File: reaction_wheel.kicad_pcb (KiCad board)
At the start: 2 copper layers, 55.7 x 65.5 mm, 33 parts, among them J1 QTH-030-01-L-D-A, J2 FTSH-105-01-L-DV, U1 TPS61379QWRTERQ1, U2 TPS62902RPJR, U8 STM32G474RETx

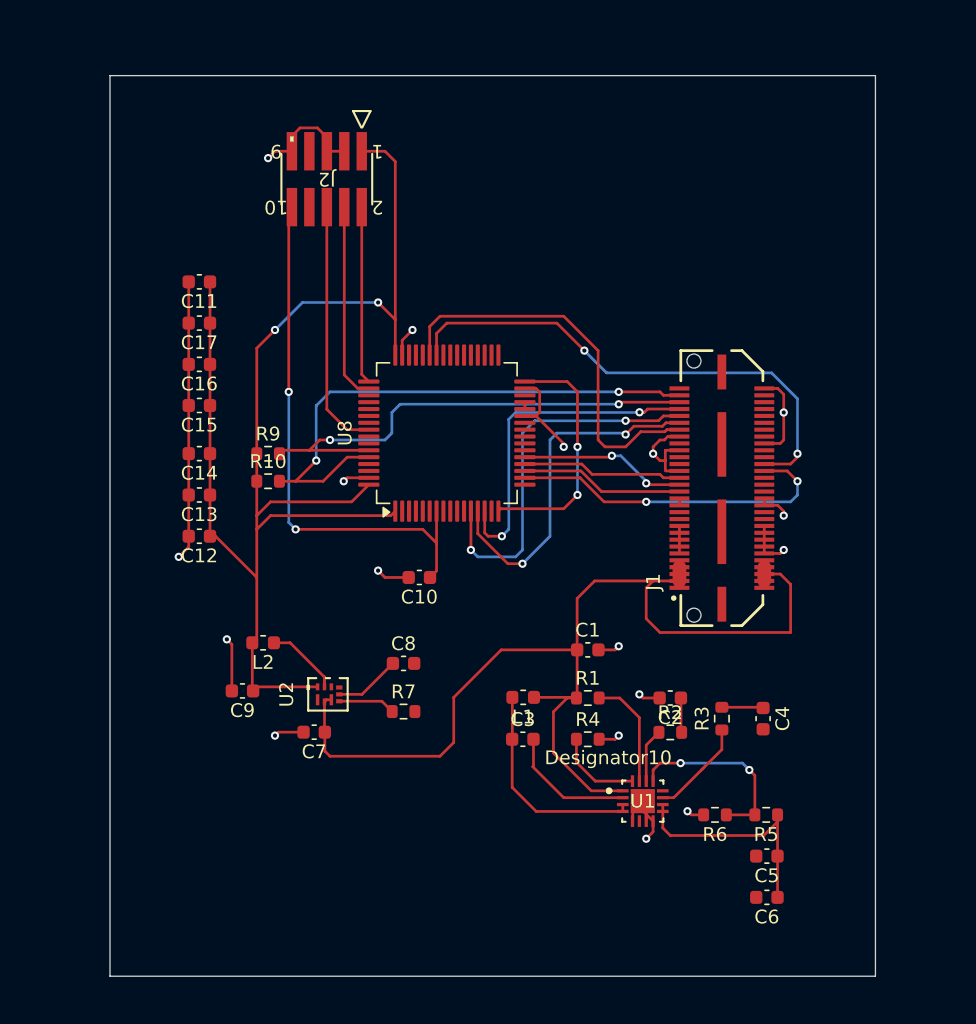
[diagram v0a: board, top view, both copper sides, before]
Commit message: finished routing, rough
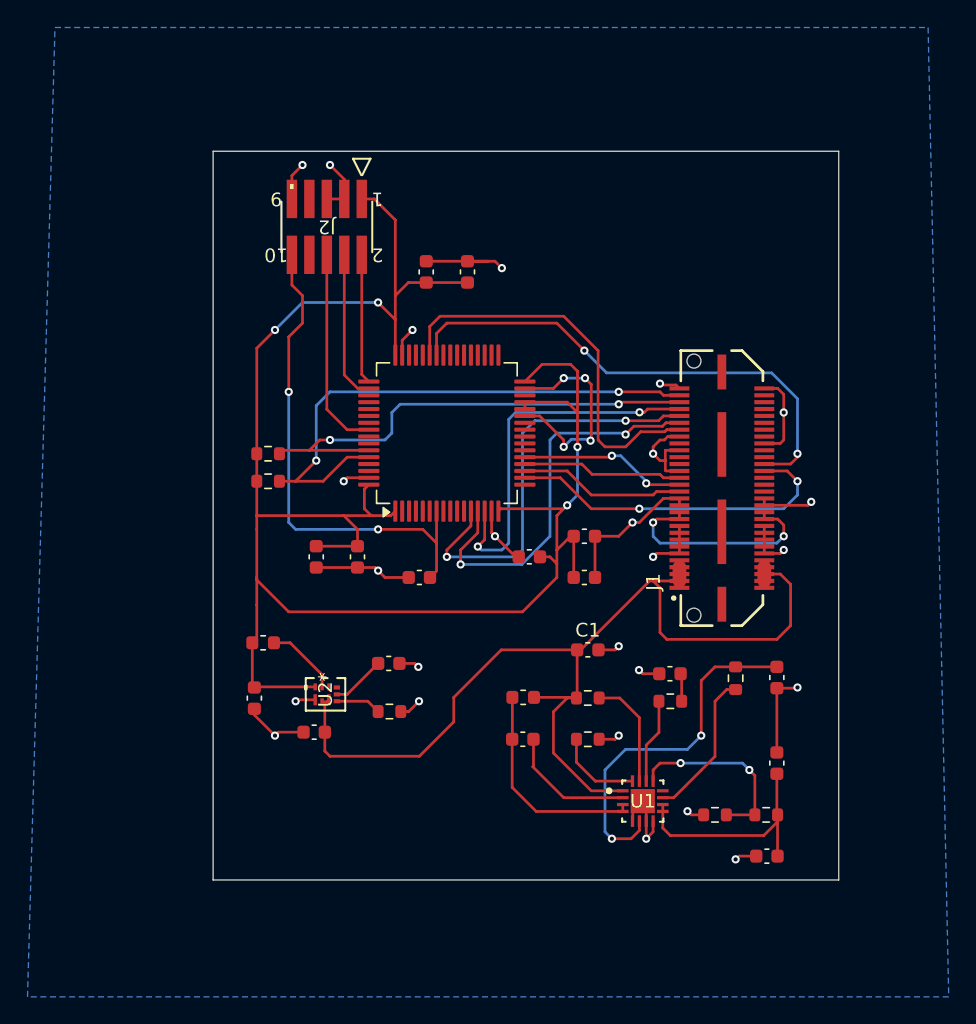
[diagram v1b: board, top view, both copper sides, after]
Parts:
- moved C11 33.6 mm to (150.5, 89.5), turned to 0 degrees
- moved C14 29.4 mm to (150.5, 92.5), turned to 0 degrees
- moved C12 27.4 mm to (142.0, 70.3), turned to 90 degrees
- moved C15 26.4 mm to (146.5, 91.0)
- moved C13 23.1 mm to (139.0, 70.3), turned to 90 degrees
- moved C17 20.5 mm to (134.0, 91.0), turned to -90 degrees
- moved C16 16.4 mm to (131.0, 91.0), turned to -90 degrees
- moved C6 9.79 mm to (164.5, 106.0), turned to 90 degrees
- moved J2 3.47 mm to (131.8, 67.0)
- moved C4 3.15 mm to (164.5, 99.8)
- moved R3 3.11 mm to (161.5, 99.8)
- moved R2 2.26 mm to (156.8, 101.5)
- moved C2 1.76 mm to (156.7, 99.5)
- moved C8 1.07 mm to (136.3, 98.8)
- moved R7 1.03 mm to (136.3, 102.2)
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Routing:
- net GND: track 82.9 -> 112.0 mm, vias 17 -> 29
- net /Power/VCC_Boost: track 3.09 -> 26.1 mm, vias 0 -> 2
- net +3V3: track 119.9 -> 138.3 mm
- net +3V3_P: track 0.00 -> 16.3 mm, vias 0 -> 2
- net /SWO: track 18.4 -> 14.9 mm
- net /SWDIO: track 12.9 -> 9.43 mm
- net /SWDCLK: track 14.4 -> 10.9 mm
- net /Power/PG_Boost: track 7.51 -> 10.9 mm
- net VBATT: track 79.0 -> 75.7 mm
- net /RW_PWR_FLT: track 25.6 -> 28.8 mm
- net /NRST: track 39.4 -> 36.6 mm
- net /RW_MTR_FLT: track 27.4 -> 30.2 mm
- net /RW_MTR_ALRM: track 24.4 -> 27.1 mm
- net /Power/COMP_Boost: track 3.93 -> 6.19 mm
- net /Power/SS_TR_Buck: track 4.83 -> 3.93 mm
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- added copper zone on B.Cu, net GND
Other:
- board size 55.7 x 65.5 mm -> 45.5 x 53 mm
